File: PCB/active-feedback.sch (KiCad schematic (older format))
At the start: 8 parts, among them U1 LM358

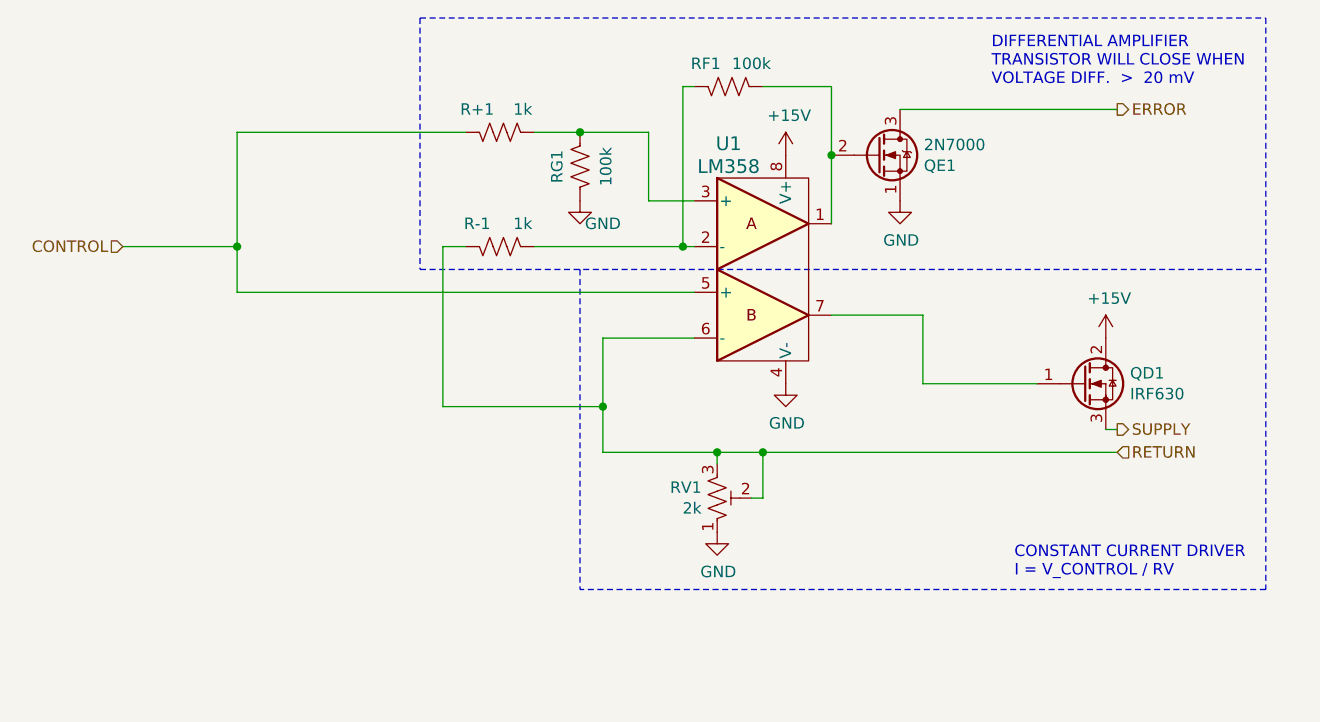
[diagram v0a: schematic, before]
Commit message: forgotten
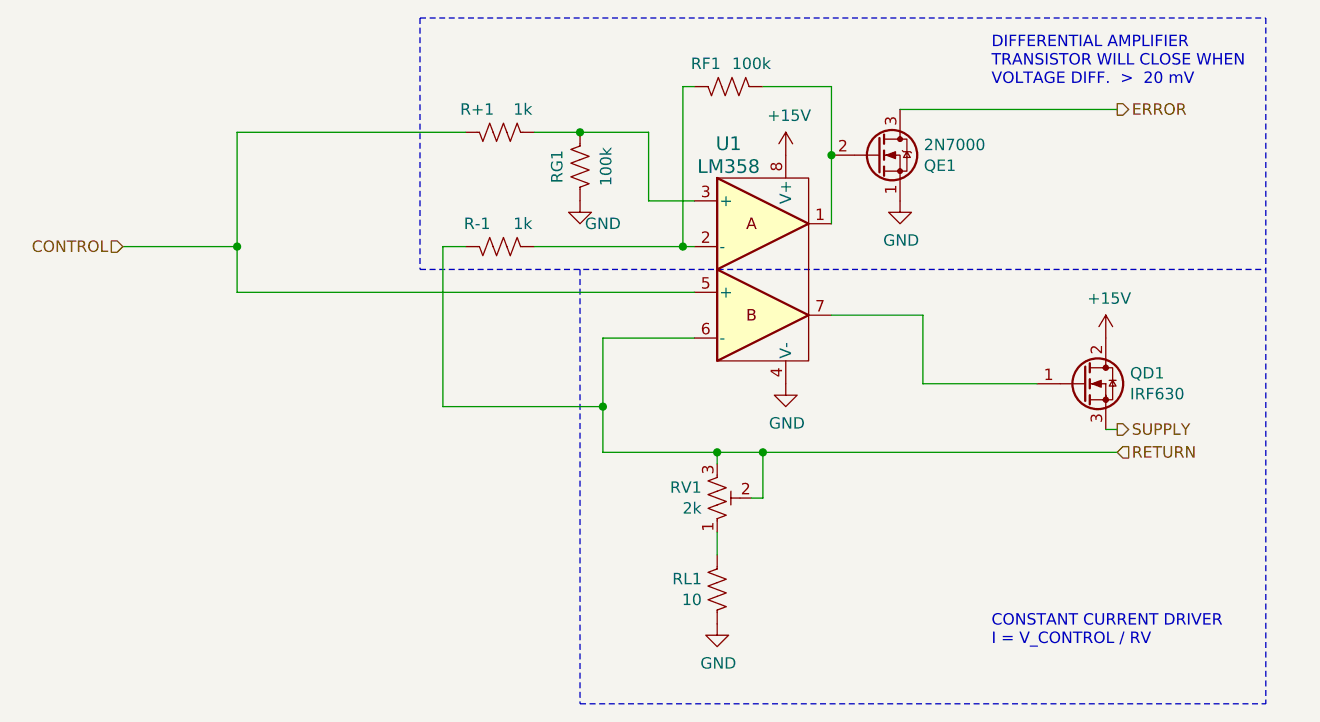
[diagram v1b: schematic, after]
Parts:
- added RL6: 10, Resistor_SMD:R_1206_3216Metric, symbol Device:R_US
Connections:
- net GND: now also RL6.1; no longer RV1.1
- new net: RL6.2, RV1.1
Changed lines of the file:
@@
 Sheet 9 9
 Title "galvanosynth"
-Date "2019-12-09"
+Date "2020-01-30"
 Rev "4.0.0"
 Comp "University of Wisconsin-Madison"
@@
 L power:GND #PWR?
 U 1 1 5E5D6B82
-P 5100 4750
+P 5100 5150
 AR Path="/5E5D6B82" Ref="#PWR?"  Part="1"
 AR Path="/5E39B760/5E5D6B82" Ref="#PWR0113"  Part="1"
@@
 AR Path="/5E3EC44B/5E5D6B82" Ref="#PWR0150"  Part="1"
 AR Path="/5E3ED540/5E5D6B82" Ref="#PWR0156"  Part="1"
-F 0 "#PWR0113" H 5100 4500 50  0001 C CNN
-F 1 "GND" H 5105 4577 50  0000 C CNN
-F 2 "" H 5100 4750 50  0001 C CNN
-F 3 "" H 5100 4750 50  0001 C CNN
-	1    5100 4750
+F 0 "#PWR0113" H 5100 4900 50  0001 C CNN
+F 1 "GND" H 5105 4977 50  0000 C CNN
+F 2 "" H 5100 5150 50  0001 C CNN
+F 3 "" H 5100 5150 50  0001 C CNN
+	1    5100 5150
 	1    0    0    -1
 $EndComp
@@
 	5300 2800 5600 2800
 $Comp
-L Device:R_US R?
+L Device:R_US R-?
 U 1 1 5E5D6BC6
 P 4150 3500
-AR Path="/5E5D6BC6" Ref="R?"  Part="1"
+AR Path="/5E5D6BC6" Ref="R-?"  Part="1"
 AR Path="/5E39B760/5E5D6BC6" Ref="R-1"  Part="1"
 AR Path="/5E3EAB60/5E5D6BC6" Ref="R-2"  Part="1"
@@
 $EndComp
 Connection ~ 5300 4400
-Wire Notes Line
-	7500 5000 4500 5000
-Wire Notes Line
-	4500 3600 4500 5000
 Wire Wire Line
 	6000 3800 6000 4100
 Wire Wire Line
 	5300 4400 6850 4400
-Text Notes 6400 4950 0    50   ~ 0
+Text Notes 6300 5250 0    50   ~ 0
 CONSTANT CURRENT DRIVER\nI = V_CONTROL / RV
 Wire Notes Line
@@
 	3800 3600 7500 3600
 $Comp
-L Device:R_US R?
+L Device:R_US R+?
 U 1 1 5E5D6BCC
 P 4150 3000
-AR Path="/5E5D6BCC" Ref="R?"  Part="1"
+AR Path="/5E5D6BCC" Ref="R+?"  Part="1"
 AR Path="/5E39B760/5E5D6BCC" Ref="R+1"  Part="1"
 AR Path="/5E3EAB60/5E5D6BCC" Ref="R+2"  Part="1"
@@
 	0    -1   1    0
 $EndComp
-Wire Notes Line
-	7500 2500 7500 5000
 Wire Notes Line
 	3800 2500 7500 2500
@@
 Connection ~ 4500 3000
 $Comp
-L Device:R_US R?
+L Device:R_US RG?
 U 1 1 5E66B3AD
 P 4500 3150
-AR Path="/5E66B3AD" Ref="R?"  Part="1"
+AR Path="/5E66B3AD" Ref="RG?"  Part="1"
 AR Path="/5E39B760/5E66B3AD" Ref="RG1"  Part="1"
 AR Path="/5E3EAB60/5E66B3AD" Ref="RG2"  Part="1"
@@
 	-1   0    0    -1
 $EndComp
+Wire Wire Line
+	5100 4750 5100 4850
+Wire Notes Line
+	4500 5500 7500 5500
+Wire Notes Line
+	4500 3600 4500 5500
+Wire Notes Line
+	7500 2500 7500 5500
+$Comp
+L Device:R_US RL6
+U 1 1 5E3668AF
+P 5100 5000
+AR Path="/5E4039E6/5E3668AF" Ref="RL6"  Part="1"
+AR Path="/5E39B760/5E3668AF" Ref="RL1"  Part="1"
+AR Path="/5E3EAB60/5E3668AF" Ref="RL2"  Part="1"
+AR Path="/5E4039EC/5E3668AF" Ref="RL7"  Part="1"
+AR Path="/5E4039F2/5E3668AF" Ref="RL8"  Part="1"
+AR Path="/5E4039E0/5E3668AF" Ref="RL5"  Part="1"
+AR Path="/5E3EC44B/5E3668AF" Ref="RL3"  Part="1"
+AR Path="/5E3ED540/5E3668AF" Ref="RL4"  Part="1"
+F 0 "RL1" H 5033 4954 50  0000 R CNN
+F 1 "10" H 5033 5045 50  0000 R CNN
+F 2 "Resistor_SMD:R_1206_3216Metric" V 5140 4990 50  0001 C CNN
+F 3 "~" H 5100 5000 50  0001 C CNN
+	1    5100 5000
+	1    0    0    1
+$EndComp
 $EndSCHEMATC
